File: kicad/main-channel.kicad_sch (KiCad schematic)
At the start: 13 parts, among them U3 TL074

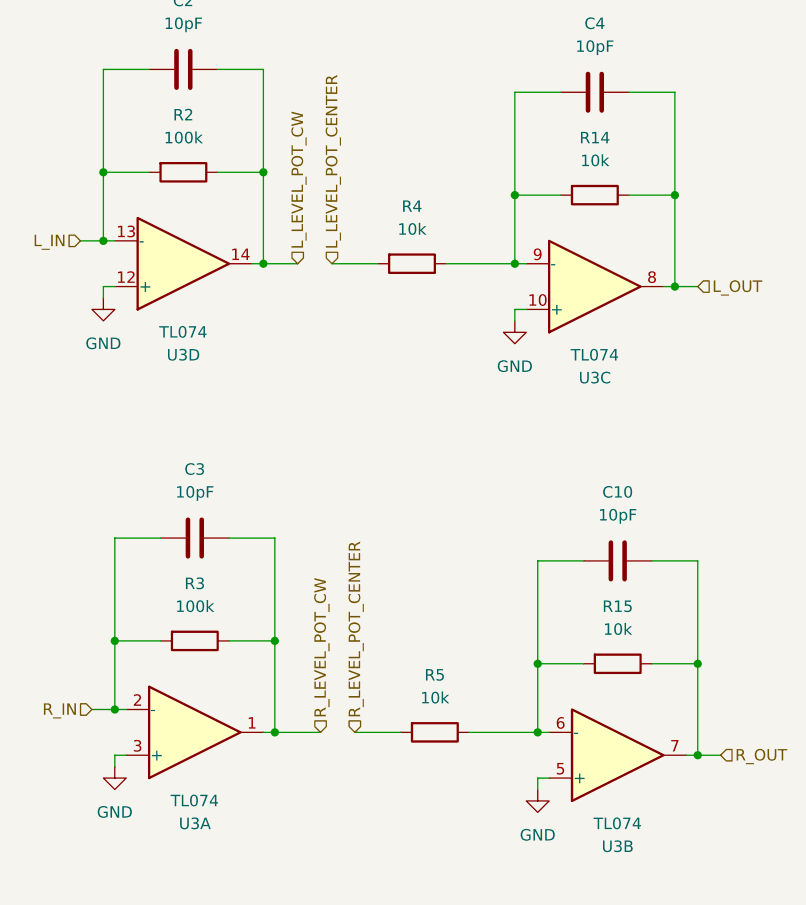
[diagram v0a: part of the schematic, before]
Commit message: Updating everything and adding gerbers
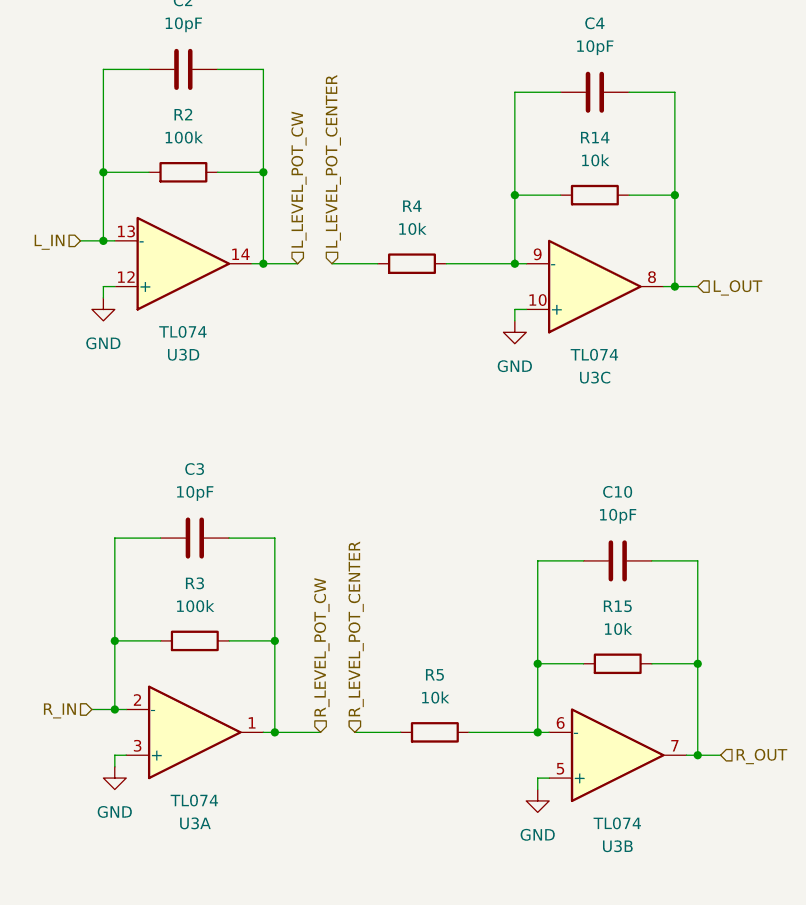
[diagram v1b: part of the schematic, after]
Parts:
- C10, C11, C12, C2, C3, C4: symbol Standard_Parts:C -> Rumblesan_Standard_Parts:C
- R14, R15, R2, R3, R4, R5: symbol Standard_Parts:R -> Rumblesan_Standard_Parts:R
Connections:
- net L_IN: now also R2.1; no longer R2.2
- net L_LEVEL_POT_CENTER: now also R4.1; no longer R4.2
- net L_LEVEL_POT_CW: now also R2.2; no longer R2.1
- net L_OUT: now also R14.2; no longer R14.1
- net R_IN: now also R3.1; no longer R3.2
- net R_LEVEL_POT_CENTER: now also R5.1; no longer R5.2
- net R_LEVEL_POT_CW: now also R3.2; no longer R3.1
- net R_OUT: now also R15.2; no longer R15.1
- net at C10.1, U3.6 (-): now also R15.1, R5.2; no longer R15.2, R5.1
- net at C4.1, U3.9 (-): now also R14.1, R4.2; no longer R14.2, R4.1
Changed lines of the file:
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@@
 	)
 	(symbol
-		(lib_id "Standard_Parts:R")
+		(lib_id "Rumblesan_Standard_Parts:R")
 		(at 93.98 97.79 90)
 		(unit 1)
@@
 	)
 	(symbol
-		(lib_id "Standard_Parts:C")
+		(lib_id "Rumblesan_Standard_Parts:C")
 		(at 111.76 26.67 90)
 		(unit 1)
@@
 	)
 	(symbol
-		(lib_id "Standard_Parts:R")
+		(lib_id "Rumblesan_Standard_Parts:R")
 		(at 114.3 90.17 90)
 		(unit 1)
@@
 	)
 	(symbol
-		(lib_id "Standard_Parts:C")
+		(lib_id "Rumblesan_Standard_Parts:C")
 		(at 223.52 93.98 180)
 		(unit 1)
@@
 	)
 	(symbol
-		(lib_id "Standard_Parts:R")
+		(lib_id "Rumblesan_Standard_Parts:R")
 		(at 66.04 35.56 90)
 		(unit 1)
@@
 	)
 	(symbol
-		(lib_id "Standard_Parts:R")
+		(lib_id "Rumblesan_Standard_Parts:R")
 		(at 67.31 87.63 90)
 		(unit 1)
@@
 	)
 	(symbol
-		(lib_id "Standard_Parts:C")
+		(lib_id "Rumblesan_Standard_Parts:C")
 		(at 67.31 76.2 90)
 		(unit 1)
@@
 	)
 	(symbol
-		(lib_id "Standard_Parts:C")
+		(lib_id "Rumblesan_Standard_Parts:C")
 		(at 114.3 78.74 90)
 		(unit 1)
@@
 	)
 	(symbol
-		(lib_id "Standard_Parts:R")
+		(lib_id "Rumblesan_Standard_Parts:R")
 		(at 111.76 38.1 90)
 		(unit 1)
@@
 	)
 	(symbol
-		(lib_id "Standard_Parts:C")
+		(lib_id "Rumblesan_Standard_Parts:C")
 		(at 223.52 106.68 180)
 		(unit 1)
@@
 	)
 	(symbol
-		(lib_id "Standard_Parts:C")
+		(lib_id "Rumblesan_Standard_Parts:C")
 		(at 66.04 24.13 90)
 		(unit 1)
@@
 	)
 	(symbol
-		(lib_id "Standard_Parts:R")
+		(lib_id "Rumblesan_Standard_Parts:R")
 		(at 91.44 45.72 90)
 		(unit 1)
